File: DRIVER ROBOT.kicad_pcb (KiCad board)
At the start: 2 copper layers, 80 x 30 mm, 103 parts, among them IC1 BTS7960B, IC2 BTS7960B, IC3 BTS7960B, IC4 BTS7960B, J1 INPUT 12V, J2 OUT MOTOR 1, J3 OUT MOTOR 2, J4 OLED 3 INCH, J5 USB_C_Receptacle_USB2.0_14P, Q1 SS8050, Q2 SS8050, SW1 RST, SW3 BOOT, U1 AMS1117-3.3, U2 ESP32-WROOM-32U, U3 HCPL-2630, U4 CH340C, U5 HCPL-2630

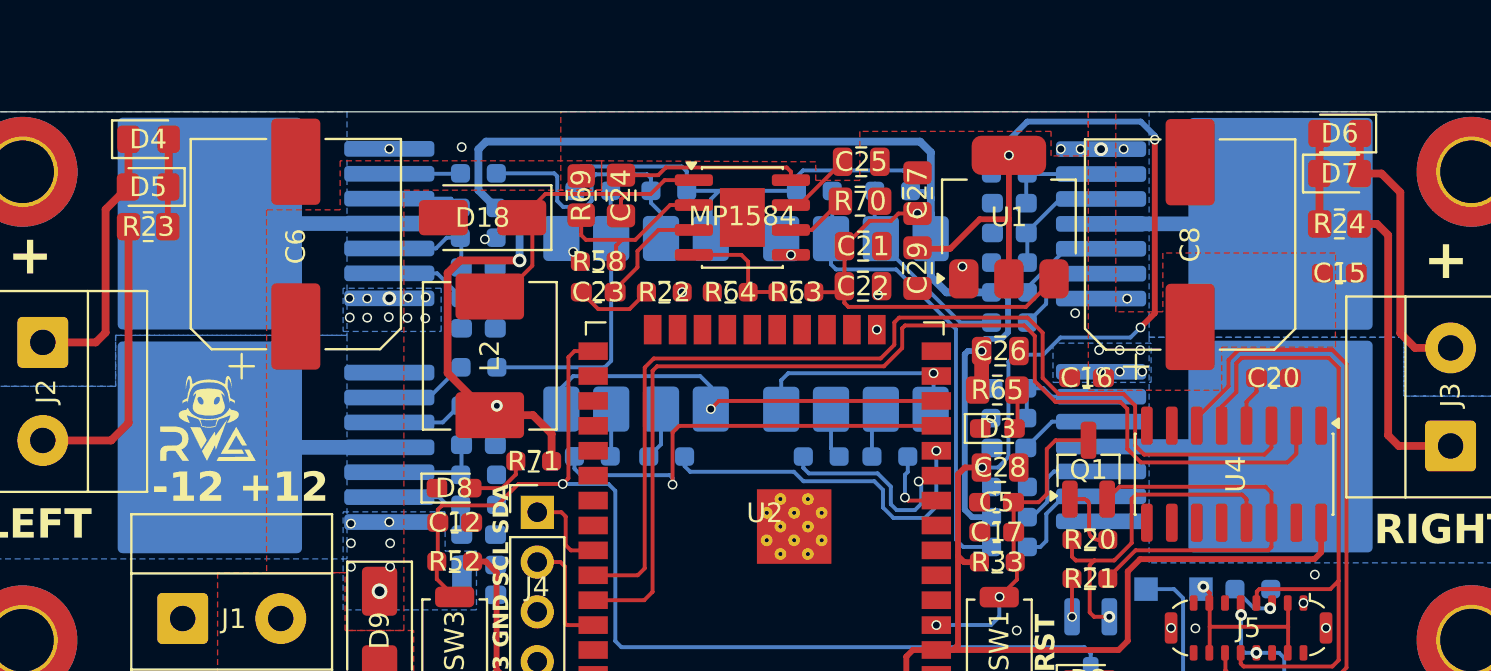
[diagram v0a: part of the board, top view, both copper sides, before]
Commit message: layout final v6
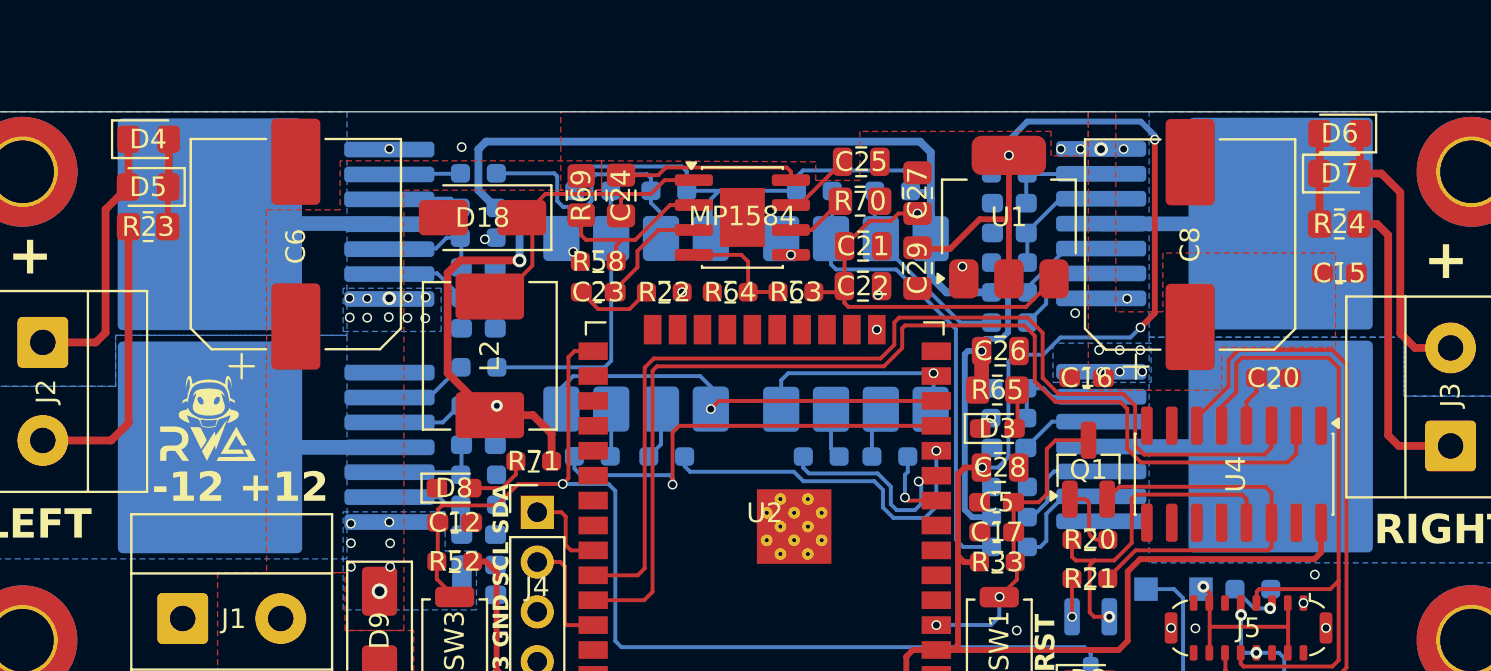
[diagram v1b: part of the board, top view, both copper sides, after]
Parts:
- removed IC1, IC2, IC3, IC4: BTS7960B, Package_TO_SOT_SMD:TO-263-7_TabPin8
- added Q3: BTN8982TA, Package_TO_SOT_SMD:TO-263-7_TabPin8, B.Cu at (113.1, 74.7)
- added Q4: BTN8982TA, Package_TO_SOT_SMD:TO-263-7_TabPin8, B.Cu at (113.1, 86.1)
- added Q7: BTN8982TA, Package_TO_SOT_SMD:TO-263-7_TabPin8, B.Cu at (164.7, 74.7)
- added Q8: BTN8982TA, Package_TO_SOT_SMD:TO-263-7_TabPin8, B.Cu at (164.7, 86.1)
